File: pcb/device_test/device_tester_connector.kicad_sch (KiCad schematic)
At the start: 8 parts, among them J201 Conn_01x05, J202 USB_C_Receptacle_USB2.0_16P, J203 Conn_01x04, J204 Conn_01x08

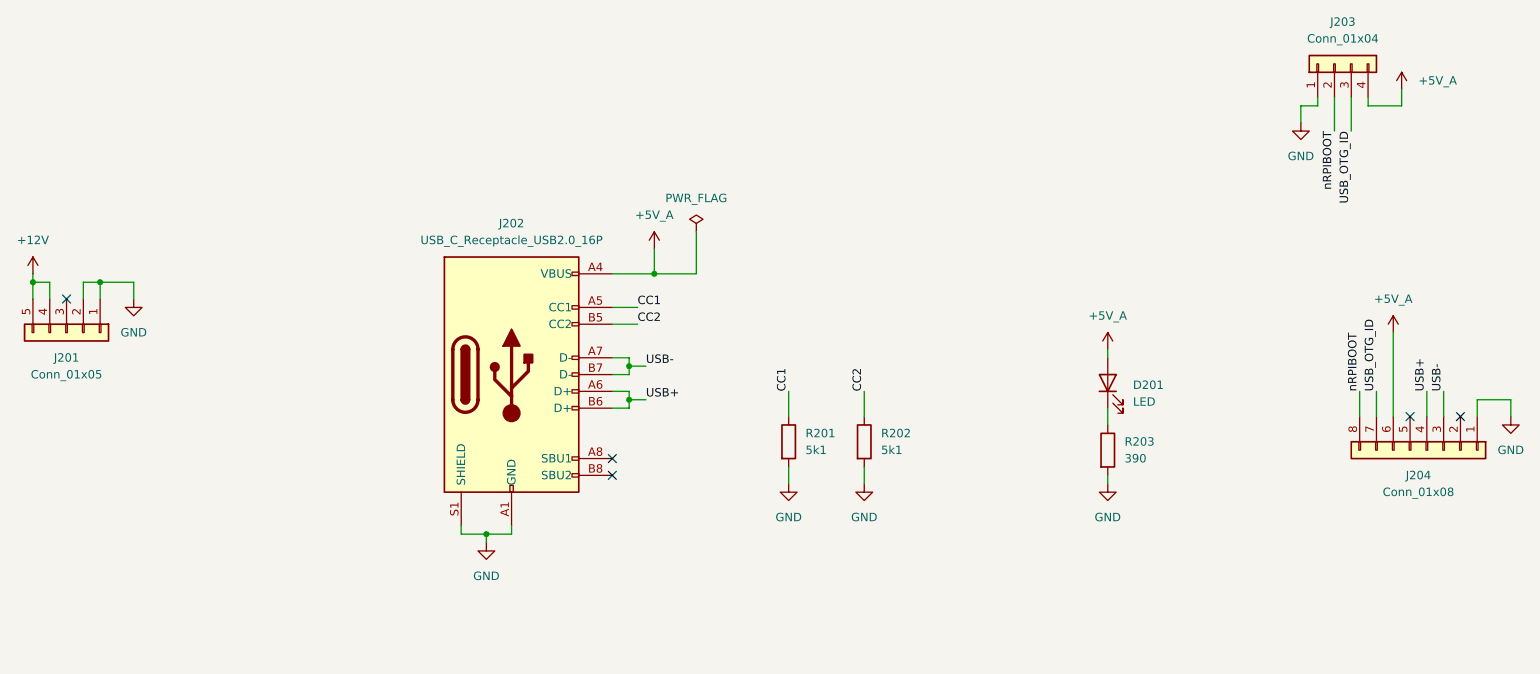
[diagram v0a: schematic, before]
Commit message: update device test pcb
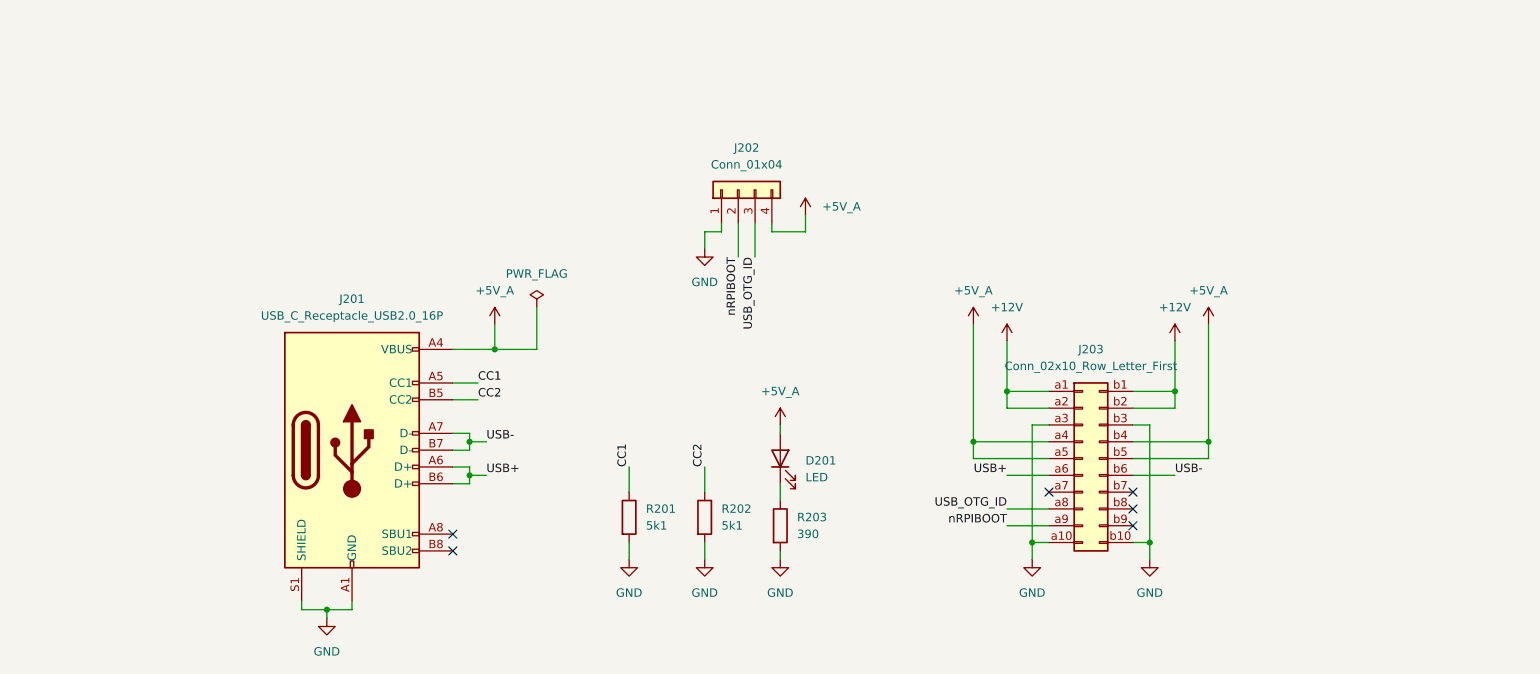
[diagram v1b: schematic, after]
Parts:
- removed J201: Conn_01x05, Connector_PinSocket_2.54mm:PinSocket_1x05_P2.54mm_Horizontal, symbol Connector_Generic:Conn_01x05
- removed J204: Conn_01x08, Connector_PinSocket_2.54mm:PinSocket_1x08_P2.54mm_Horizontal, symbol Connector_Generic:Conn_01x08
- added J203: Conn_02x10_Row_Letter_First, Connector_DIN:DIN41612_B3_2x10_Male_Horizontal_THT, symbol Connector_Generic:Conn_02x10_Row_Letter_First
- renumbered J202 to J201, J203 to J202
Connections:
- net +12V: now also J203.a1 (Pin_a1), J203.a2 (Pin_a2), J203.b1 (Pin_b1), J203.b2 (Pin_b2)
- net +5V_A: now also J203.a4 (Pin_a4), J203.a5 (Pin_a5), J203.b4 (Pin_b4), J203.b5 (Pin_b5)
- net GND: now also J203.a10 (Pin_a10), J203.a3 (Pin_a3), J203.b10 (Pin_b10), J203.b3 (Pin_b3)
- net USB+: now also J203.a6 (Pin_a6)
- net USB-: now also J203.b6 (Pin_b6)
- net USB_OTG_ID: now also J203.a8 (Pin_a8)
- net nRPIBOOT: now also J203.a9 (Pin_a9)
- no-connect marks 5 -> 6
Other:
- moved on the sheet: D201, J201, J202, R201, R202, R203
